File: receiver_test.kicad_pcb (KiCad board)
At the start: 2 copper layers, 58 parts, among them J1 RF_IN, J2 IF_IN, J3 Conn_01x02_Male, J4 Conn_01x02_Male, J6 5V, Q1 MMBT5089, Q2 BC847BS, U1 ADE-1H+, U2 SA612, U3 MCP6D11, U4 FST3253, Y1 28.636 MHz

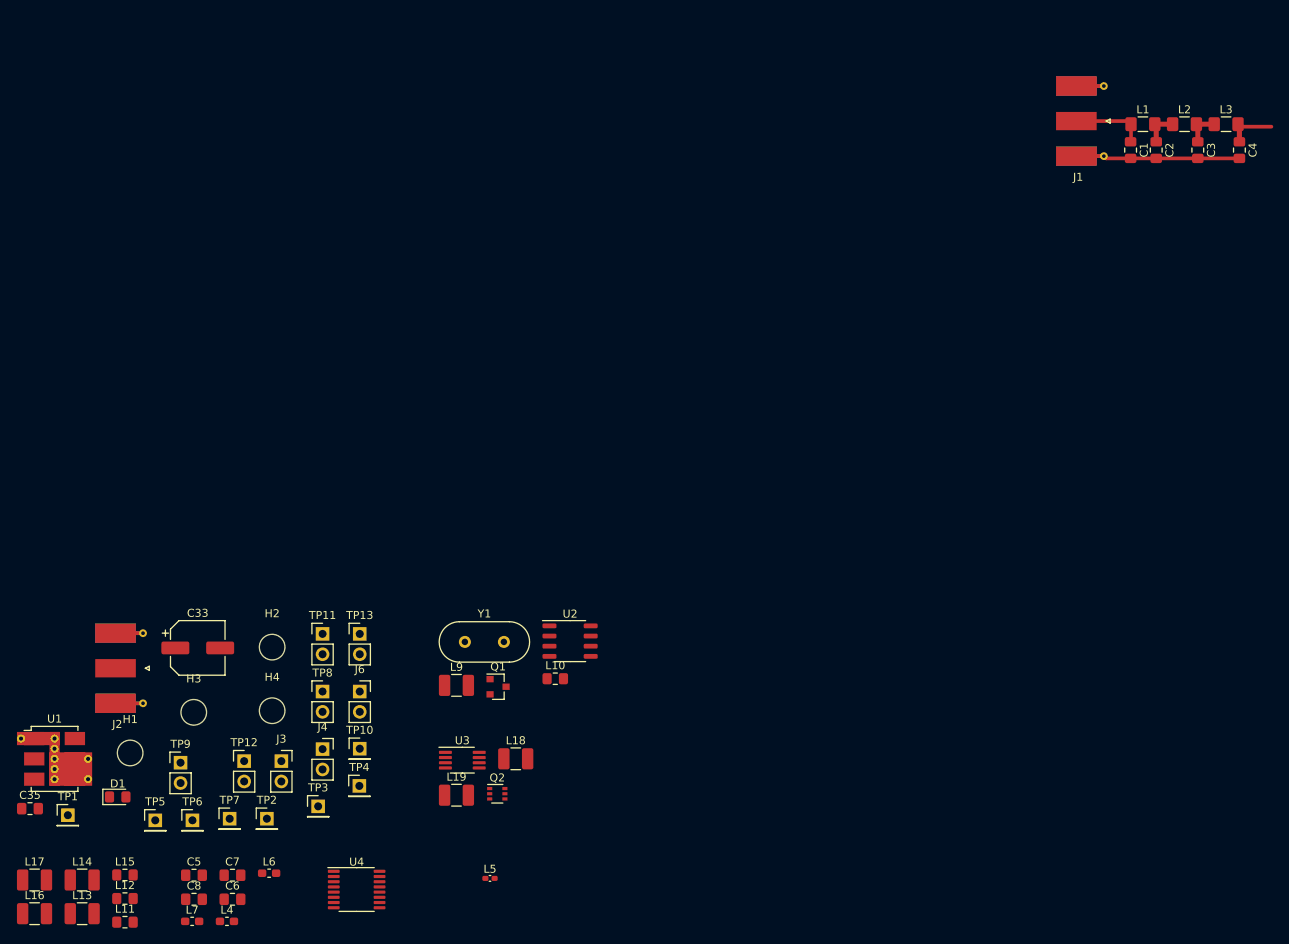
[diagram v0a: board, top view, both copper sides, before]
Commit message: Pcb vHA8KDA
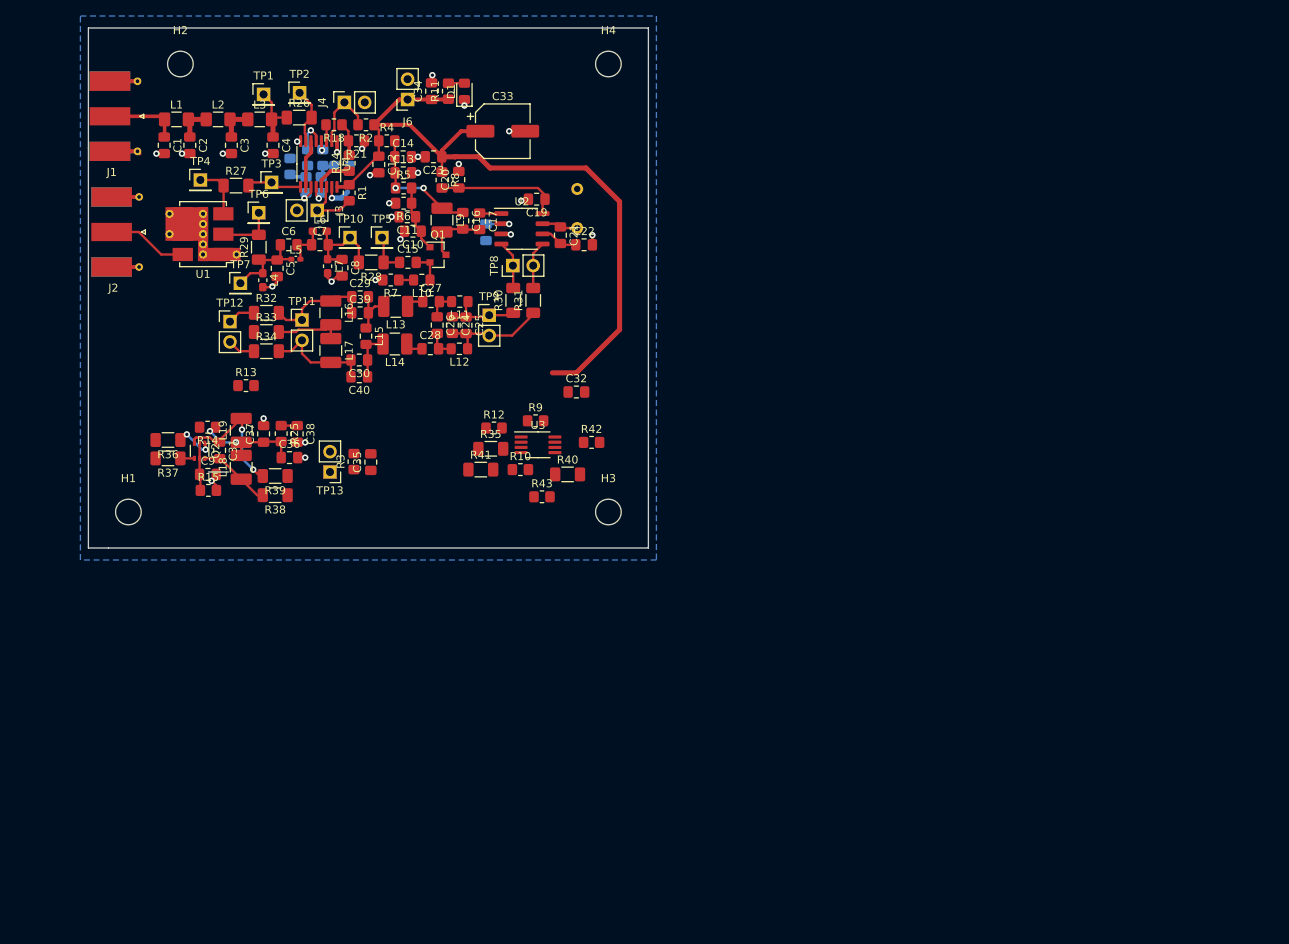
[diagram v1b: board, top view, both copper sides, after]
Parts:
- added C10: 10n, Capacitor_SMD:C_0805_2012Metric_Pad1.18x1.45mm_HandSolder, F.Cu at (75.6, 97.9)
- added C11: 100n, Capacitor_SMD:C_0805_2012Metric_Pad1.18x1.45mm_HandSolder, F.Cu at (74.9, 96.1)
- added C12: 100n, Capacitor_SMD:C_0805_2012Metric_Pad1.18x1.45mm_HandSolder, F.Cu at (71.3, 89.6)
- added C13: 100n, Capacitor_SMD:C_0805_2012Metric_Pad1.18x1.45mm_HandSolder, F.Cu at (74.4, 90.6)
- added C14: 10n, Capacitor_SMD:C_0805_2012Metric_Pad1.18x1.45mm_HandSolder, F.Cu at (74.3, 88.6)
- added C15: 10n, Capacitor_SMD:C_0805_2012Metric_Pad1.18x1.45mm_HandSolder, F.Cu at (74.9, 101.8)
- added C16: 100p, Capacitor_SMD:C_0805_2012Metric_Pad1.18x1.45mm_HandSolder, F.Cu at (81.8, 96.6)
- added C17: 10n, Capacitor_SMD:C_0805_2012Metric_Pad1.18x1.45mm_HandSolder, F.Cu at (83.9, 96.7)
- added C18: 10n, Capacitor_SMD:C_0805_2012Metric_Pad1.18x1.45mm_HandSolder, B.Cu at (84.7, 98.0)
- added C19: 10n, Capacitor_SMD:C_0805_2012Metric_Pad1.18x1.45mm_HandSolder, F.Cu at (91.0, 93.9)
- added C20: 100n, Capacitor_SMD:C_0805_2012Metric_Pad1.18x1.45mm_HandSolder, F.Cu at (81.3, 91.5)
- added C21: 36p, Capacitor_SMD:C_0805_2012Metric_Pad1.18x1.45mm_HandSolder, F.Cu at (94.0, 98.4)
- added C22: 36p, Capacitor_SMD:C_0805_2012Metric_Pad1.18x1.45mm_HandSolder, F.Cu at (97.0, 99.6)
- added C23: 100n, Capacitor_SMD:C_0805_2012Metric_Pad1.18x1.45mm_HandSolder, F.Cu at (78.1, 88.6)
- added C24: 68p, Capacitor_SMD:C_0805_2012Metric_Pad1.18x1.45mm_HandSolder, F.Cu at (80.5, 109.6)
- added C25: 15p, Capacitor_SMD:C_0805_2012Metric_Pad1.18x1.45mm_HandSolder, F.Cu at (82.2, 109.7)
- added C26: 470p, Capacitor_SMD:C_0805_2012Metric_Pad1.18x1.45mm_HandSolder, F.Cu at (78.6, 109.6)
- added C27: 18p, Capacitor_SMD:C_0805_2012Metric_Pad1.18x1.45mm_HandSolder, F.Cu at (77.8, 106.7)
- added C28: 18p, Capacitor_SMD:C_0805_2012Metric_Pad1.18x1.45mm_HandSolder, F.Cu at (77.7, 112.6)
- added C29: 180p, Capacitor_SMD:C_0805_2012Metric_Pad1.18x1.45mm_HandSolder, F.Cu at (69.0, 106.1)
- added C30: 180p, Capacitor_SMD:C_0805_2012Metric_Pad1.18x1.45mm_HandSolder, F.Cu at (68.9, 114.0)
- added C31: 9p, Capacitor_SMD:C_0805_2012Metric_Pad1.18x1.45mm_HandSolder, F.Cu at (51.4, 125.3)
- added C32: 10n, Capacitor_SMD:C_0805_2012Metric_Pad1.18x1.45mm_HandSolder, F.Cu at (96.0, 118.0)
- added C34: 100n, Capacitor_SMD:C_0805_2012Metric_Pad1.18x1.45mm_HandSolder, F.Cu at (77.9, 80.4)
- added C36: 10n, Capacitor_SMD:C_0805_2012Metric_Pad1.18x1.45mm_HandSolder, F.Cu at (60.1, 126.2)
- added C37: 100n, Capacitor_SMD:C_0805_2012Metric_Pad1.18x1.45mm_HandSolder, F.Cu at (56.9, 123.2)
- added C38: 100n, Capacitor_SMD:C_0805_2012Metric_Pad1.18x1.45mm_HandSolder, F.Cu at (61.1, 123.2)
- added C39: 33p, Capacitor_SMD:C_0805_2012Metric_Pad1.18x1.45mm_HandSolder, F.Cu at (69.0, 108.1)
- added C40: 33p, Capacitor_SMD:C_0805_2012Metric_Pad1.18x1.45mm_HandSolder, F.Cu at (68.9, 116.1)
- added C9: 10n, Capacitor_SMD:C_0805_2012Metric_Pad1.18x1.45mm_HandSolder, F.Cu at (49.9, 128.3)
- added R1: 5k, Resistor_SMD:R_0805_2012Metric_Pad1.20x1.40mm_HandSolder, F.Cu at (67.6, 93.1)
- added R10: 1.2k, Resistor_SMD:R_0805_2012Metric_Pad1.20x1.40mm_HandSolder, F.Cu at (89.0, 127.7)
- added R11: 470, Resistor_SMD:R_0805_2012Metric_Pad1.20x1.40mm_HandSolder, F.Cu at (80.0, 80.4)
- added R12: BP, Resistor_SMD:R_0805_2012Metric_Pad1.20x1.40mm_HandSolder, F.Cu at (85.7, 122.5)
- added R13: 2k5, Resistor_SMD:R_0805_2012Metric_Pad1.20x1.40mm_HandSolder, F.Cu at (54.7, 117.2)
- added R14: 19k, Resistor_SMD:R_0805_2012Metric_Pad1.20x1.40mm_HandSolder, F.Cu at (49.9, 122.4)
- added R15: 31k, Resistor_SMD:R_0805_2012Metric_Pad1.20x1.40mm_HandSolder, F.Cu at (50.0, 130.3)
- added R16: 27, Resistor_SMD:R_0805_2012Metric_Pad1.20x1.40mm_HandSolder, B.Cu at (62.4, 88.7)
- added R17: 39, Resistor_SMD:R_0805_2012Metric_Pad1.20x1.40mm_HandSolder, B.Cu at (64.3, 88.7)
- added R18: 47, Resistor_SMD:R_0805_2012Metric_Pad1.20x1.40mm_HandSolder, F.Cu at (65.7, 84.6)
- added R19: 33, Resistor_SMD:R_0805_2012Metric_Pad1.20x1.40mm_HandSolder, B.Cu at (60.2, 89.8)
- added R2: 5k, Resistor_SMD:R_0805_2012Metric_Pad1.20x1.40mm_HandSolder, F.Cu at (69.7, 84.6)
- added R20: 10, Resistor_SMD:R_0805_2012Metric_Pad1.20x1.40mm_HandSolder, B.Cu at (66.7, 89.8)
- added R21: 3, Resistor_SMD:R_0805_2012Metric_Pad1.20x1.40mm_HandSolder, F.Cu at (68.5, 86.6)
- added R22: 27, Resistor_SMD:R_0805_2012Metric_Pad1.20x1.40mm_HandSolder, B.Cu at (62.2, 92.1)
- added R23: 39, Resistor_SMD:R_0805_2012Metric_Pad1.20x1.40mm_HandSolder, B.Cu at (64.1, 92.1)
- added R24: 47, Resistor_SMD:R_0805_2012Metric_Pad1.20x1.40mm_HandSolder, F.Cu at (67.6, 89.4)
- added R25: 100, Resistor_SMD:R_0805_2012Metric_Pad1.20x1.40mm_HandSolder, F.Cu at (59.1, 123.2)
- added R26: BP, Resistor_SMD:R_1206_3216Metric_Pad1.30x1.75mm_HandSolder, F.Cu at (61.4, 83.7)
- added R27: BP, Resistor_SMD:R_1206_3216Metric_Pad1.30x1.75mm_HandSolder, F.Cu at (53.5, 92.2)
- added R28: BP, Resistor_SMD:R_1206_3216Metric_Pad1.30x1.75mm_HandSolder, F.Cu at (70.3, 101.8)
- added R29: BP, Resistor_SMD:R_1206_3216Metric_Pad1.30x1.75mm_HandSolder, F.Cu at (56.3, 99.9)
- added R3: 10k, Resistor_SMD:R_0805_2012Metric_Pad1.20x1.40mm_HandSolder, F.Cu at (68.2, 126.7)
- added R30: BP, Resistor_SMD:R_1206_3216Metric_Pad1.30x1.75mm_HandSolder, F.Cu at (88.1, 106.5)
- added R31: BP, Resistor_SMD:R_1206_3216Metric_Pad1.30x1.75mm_HandSolder, F.Cu at (90.6, 106.5)
- added R32: BP, Resistor_SMD:R_1206_3216Metric_Pad1.30x1.75mm_HandSolder, F.Cu at (57.2, 108.1)
- added R33: BP, Resistor_SMD:R_1206_3216Metric_Pad1.30x1.75mm_HandSolder, F.Cu at (57.2, 110.5)
- added R34: BP, Resistor_SMD:R_1206_3216Metric_Pad1.30x1.75mm_HandSolder, F.Cu at (57.2, 112.9)
- added R35: BP, Resistor_SMD:R_1206_3216Metric_Pad1.30x1.75mm_HandSolder, F.Cu at (85.3, 125.1)
- added R36: BP, Resistor_SMD:R_1206_3216Metric_Pad1.30x1.75mm_HandSolder, F.Cu at (45.0, 124.0)
- added R37: BP, Resistor_SMD:R_1206_3216Metric_Pad1.30x1.75mm_HandSolder, F.Cu at (45.0, 126.3)
- added R38: BP, Resistor_SMD:R_1206_3216Metric_Pad1.30x1.75mm_HandSolder, F.Cu at (58.4, 130.9)
- added R39: BP, Resistor_SMD:R_1206_3216Metric_Pad1.30x1.75mm_HandSolder, F.Cu at (58.4, 128.5)
- added R4: 100, Resistor_SMD:R_0805_2012Metric_Pad1.20x1.40mm_HandSolder, F.Cu at (72.3, 86.6)
- added R40: BP, Resistor_SMD:R_1206_3216Metric_Pad1.30x1.75mm_HandSolder, F.Cu at (94.9, 128.3)
- added R41: BP, Resistor_SMD:R_1206_3216Metric_Pad1.30x1.75mm_HandSolder, F.Cu at (84.0, 127.7)
- added R42: 19k, Resistor_SMD:R_0805_2012Metric_Pad1.20x1.40mm_HandSolder, F.Cu at (97.9, 124.3)
- added R43: 19k, Resistor_SMD:R_0805_2012Metric_Pad1.20x1.40mm_HandSolder, F.Cu at (91.7, 131.1)
- added R5: 28k, Resistor_SMD:R_0805_2012Metric_Pad1.20x1.40mm_HandSolder, F.Cu at (74.4, 92.5)
- added R6: 31k, Resistor_SMD:R_0805_2012Metric_Pad1.20x1.40mm_HandSolder, F.Cu at (74.4, 94.4)
- added R7: 5k, Resistor_SMD:R_0805_2012Metric_Pad1.20x1.40mm_HandSolder, F.Cu at (72.8, 104.0)
- added R8: 100, Resistor_SMD:R_0805_2012Metric_Pad1.20x1.40mm_HandSolder, F.Cu at (79.2, 91.5)
- added R9: 1.2k, Resistor_SMD:R_0805_2012Metric_Pad1.20x1.40mm_HandSolder, F.Cu at (90.9, 121.6)
- Y1: moved to B.Cu
- moved C1 120.8 mm to (44.5, 87.2)
- moved C4 120.8 mm to (58.1, 87.2)
- moved J1 120.8 mm to (39.4, 83.5)
- moved L1 120.8 mm to (46.0, 83.9)
- moved L3 120.8 mm to (56.4, 83.9)
- moved C2 120.8 mm to (47.7, 87.2)
- moved C3 120.8 mm to (52.9, 87.2)
- moved L2 120.8 mm to (51.2, 83.9)
- moved D1 98.3 mm to (82.0, 80.4), turned to 90 degrees
- moved TP1 93.4 mm to (56.9, 80.8)
- moved H4 91.1 mm to (100.0, 77.0)
- moved TP2 90.8 mm to (61.4, 80.6)
- moved U4 90.8 mm to (63.8, 89.5), turned to 270 degrees
- moved L11 88.1 mm to (81.4, 106.7), turned to 180 degrees
- moved L13 85.4 mm to (73.4, 107.3), turned to 180 degrees
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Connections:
- D1 pad 2: (no net) -> Net-(D1-Pad2)
- L10 pad 2: (no net) -> Net-(L10-Pad2)
- L11 pad 2: (no net) -> Net-(C26-Pad1)
- L12 pad 2: (no net) -> Net-(C26-Pad2)
- L13 pad 1: (no net) -> Net-(C27-Pad1)
- L14 pad 1: (no net) -> Net-(C28-Pad1)
- L9 pad 1: (no net) -> Net-(C13-Pad1)
- Q1 pad 1: (no net) -> Net-(C10-Pad1)
- Q2 pad 1: (no net) -> Net-(Q2-Pad1)
- Q2 pad 4: (no net) -> Net-(Q2-Pad4)
- TP12 pad 1: (no net) -> /Sheet5FE3342E/In+
- TP12 pad 2: (no net) -> /Sheet5FE3342E/In-
- TP5 pad 1: (no net) -> /37.4 MHz Amp, and 2nd mixer/IN
- U2 pad 1: (no net) -> Net-(C17-Pad1)
- U2 pad 2: (no net) -> Net-(C18-Pad1)
- U2 pad 6: (no net) -> Net-(C21-Pad2)
- U2 pad 8: (no net) -> Net-(C19-Pad1)
- U3 pad 1: (no net) -> Net-(R10-Pad2)
- U3 pad 2: (no net) -> /Sheet5FE3342E/DC_CM
- U3 pad 4: (no net) -> Net-(R40-Pad2)
- U3 pad 5: (no net) -> Net-(R10-Pad1)
- U3 pad 6: (no net) -> GND
- U3 pad 8: (no net) -> Net-(R12-Pad1)
- U4 pad 11: (no net) -> /Attenuator/10dB_out
- U4 pad 12: (no net) -> /Attenuator/20dB_out
- U4 pad 13: (no net) -> /Attenuator/30dB_out
- U4 pad 3: (no net) -> /Attenuator/30dB_in
- U4 pad 4: (no net) -> /Attenuator/20dB_in
- U4 pad 5: (no net) -> /Attenuator/10dB_in
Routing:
- net +5VA: track 0.00 -> 93.4 mm
- net GNDA: track 23.9 -> 44.5 mm, vias 0 -> 28
- net Net-(C31-Pad1): track 0.00 -> 16.6 mm, vias 0 -> 2
- net Net-(C13-Pad1): track 0.00 -> 15.7 mm, vias 0 -> 2
- net Net-(C19-Pad1): track 0.00 -> 15.7 mm
- net /Sheet5FE333A0/Out-: track 0.00 -> 13.9 mm
- net /Sheet5FE333A0/In-: track 0.00 -> 13.5 mm
- net /Sheet5FE333A0/Out+: track 0.00 -> 13.5 mm
- net Net-(C36-Pad1): track 0.00 -> 13.4 mm, vias 0 -> 2
- net /37.4 MHz BPF/OUT: track 0.00 -> 12.2 mm
- net /37.4 MHz BPF/IN: track 0.00 -> 11.5 mm
- net Net-(J2-Pad1): track 0.00 -> 10.1 mm
- net /Sheet5FE333A0/In+: track 0.00 -> 9.63 mm
- net Net-(C31-Pad2): track 0.00 -> 9.16 mm
- net /Attenuator/ATT_SEL1: track 0.00 -> 8.99 mm
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- added copper zone on B.Cu, net GNDA
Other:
- board outline added: 70 x 65 mm
